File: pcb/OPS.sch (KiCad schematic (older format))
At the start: 45 parts, among them P10 2SC3281, P11 2SC3281, P12 2SA1302, P7 MJE350, P8 MJE340, P9 2SA1302, Q13 MPSA56_PNP_EBC, Q14 MPSA06_NPN_EBC, Q15 MPSA56_PNP_EBC, Q16 MPSA06_NPN_EBC, Q17 MJE340_NPN_ECB, Q18 MJE350_PNP_EBC, Q19 MJE340_NPN_ECB, Q20 MJE350_PNP_EBC

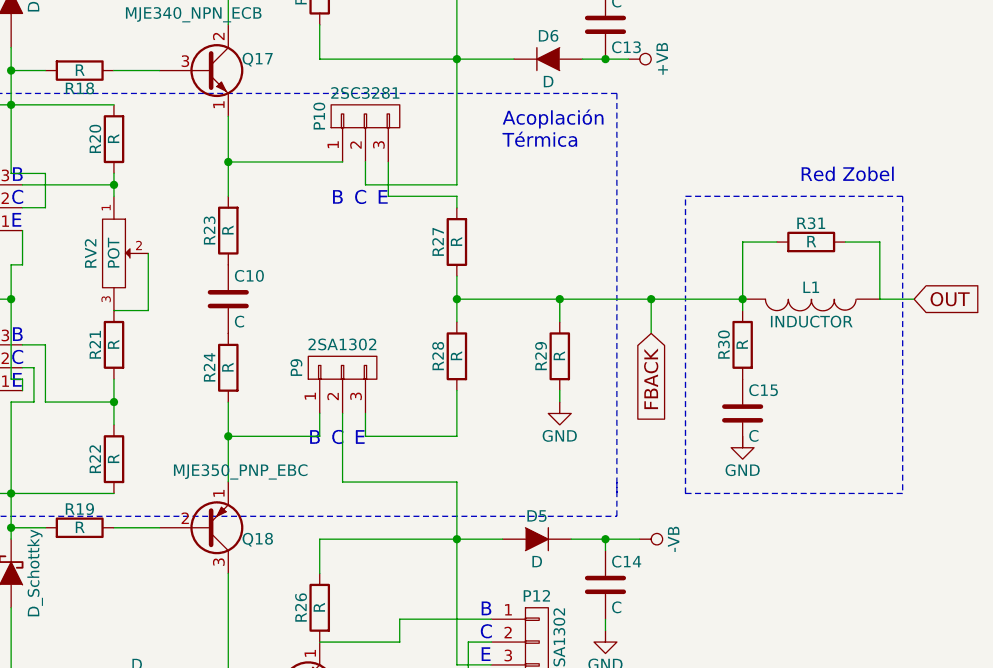
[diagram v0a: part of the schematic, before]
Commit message: ultimos avances falta poco para terminar
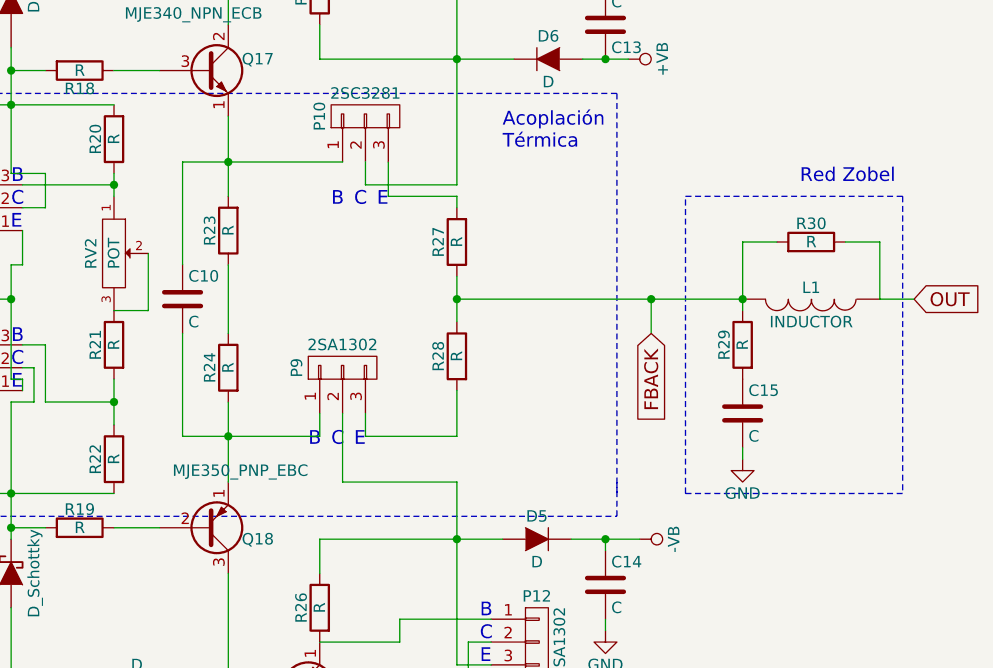
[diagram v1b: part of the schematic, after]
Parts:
- removed R29: R, Resistors_ThroughHole:Resistor_Horizontal_RM10mm, symbol R
- renumbered R30 to R29, R31 to R30
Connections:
- net GND: now also C15.2
- net at R23.1: now also R24.1; no longer C10.1
- net at P10.1 (P1), Q17.1 (E), R23.2: now also C10.1
- net at C10.2: now also P9.1 (P1), Q18.1 (E), R24.2; no longer R24.1
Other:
- moved on the sheet: C10
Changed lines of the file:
@@
 Text GLabel 3450 3550 0    60   Input ~ 0
 TO_OPS
-$Comp
-L R R29
-U 1 1 555E676F
-P 6400 3800
-F 0 "R29" V 6480 3800 50  0000 C CNN
-F 1 "R" V 6400 3800 50  0000 C CNN
-F 2 "Resistors_ThroughHole:Resistor_Horizontal_RM10mm" V 6330 3800 30  0001 C CNN
-F 3 "" H 6400 3800 30  0000 C CNN
-	1    6400 3800
-	-1   0    0    -1
-$EndComp
-$Comp
-L GND #PWR031
-U 1 1 555E69E7
-P 6400 4000
-F 0 "#PWR031" H 6400 3750 50  0001 C CNN
-F 1 "GND" H 6400 3850 50  0000 C CNN
-F 2 "" H 6400 4000 60  0000 C CNN
-F 3 "" H 6400 4000 60  0000 C CNN
-	1    6400 4000
-	1    0    0    -1
-$EndComp
 Text GLabel 6800 3700 3    60   Input ~ 0
 FBACK
 $Comp
-L GND #PWR032
+L GND #PWR031
 U 1 1 555F209B
 P 3200 5050
-F 0 "#PWR032" H 3200 4800 50  0001 C CNN
+F 0 "#PWR031" H 3200 4800 50  0001 C CNN
 F 1 "GND" H 3200 4900 50  0000 C CNN
 F 2 "" H 3200 5050 60  0000 C CNN
@@
 $EndComp
 $Comp
-L GND #PWR033
+L GND #PWR032
 U 1 1 555E698A
 P 3200 2100
-F 0 "#PWR033" H 3200 1850 50  0001 C CNN
+F 0 "#PWR032" H 3200 1850 50  0001 C CNN
 F 1 "GND" H 3200 1950 50  0000 C CNN
 F 2 "" H 3200 2100 60  0000 C CNN
@@
 $EndComp
 $Comp
-L +VA #PWR034
+L +VA #PWR033
 U 1 1 555F2B00
 P 6300 900
-F 0 "#PWR034" H 6300 750 50  0001 C CNN
+F 0 "#PWR033" H 6300 750 50  0001 C CNN
 F 1 "+VA" H 6300 1050 50  0000 C CNN
 F 2 "" H 6300 900 60  0000 C CNN
@@
 $EndComp
 $Comp
-L +VB #PWR035
+L +VB #PWR034
 U 1 1 555F2D0C
 P 6700 2500
-F 0 "#PWR035" H 6700 2350 50  0001 C CNN
+F 0 "#PWR034" H 6700 2350 50  0001 C CNN
 F 1 "+VB" H 6700 2650 50  0000 C CNN
 F 2 "" H 6700 2500 60  0000 C CNN
@@
 $EndComp
 $Comp
-L -VB #PWR036
+L -VB #PWR035
 U 1 1 555F3146
 P 6750 4600
-F 0 "#PWR036" H 6750 4450 50  0001 C CNN
+F 0 "#PWR035" H 6750 4450 50  0001 C CNN
 F 1 "-VB" H 6750 4750 50  0000 C CNN
 F 2 "" H 6750 4600 60  0000 C CNN
@@
 $EndComp
 $Comp
-L -VA #PWR037
+L -VA #PWR036
 U 1 1 555F3328
 P 6300 6200
-F 0 "#PWR037" H 6300 6050 50  0001 C CNN
+F 0 "#PWR036" H 6300 6050 50  0001 C CNN
 F 1 "-VA" H 6300 6350 50  0000 C CNN
 F 2 "" H 6300 6200 60  0000 C CNN
@@
 $EndComp
 $Comp
-L GND #PWR038
+L GND #PWR037
 U 1 1 556CC8CC
 P 5750 5750
-F 0 "#PWR038" H 5750 5500 50  0001 C CNN
+F 0 "#PWR037" H 5750 5500 50  0001 C CNN
 F 1 "GND" H 5750 5600 50  0000 C CNN
 F 2 "" H 5750 5750 60  0000 C CNN
@@
 $EndComp
 $Comp
-L GND #PWR039
+L GND #PWR038
 U 1 1 556CCB94
 P 6150 1300
-F 0 "#PWR039" H 6150 1050 50  0001 C CNN
+F 0 "#PWR038" H 6150 1050 50  0001 C CNN
 F 1 "GND" H 6150 1150 50  0000 C CNN
 F 2 "" H 6150 1300 60  0000 C CNN
@@
 $EndComp
 $Comp
-L GND #PWR040
+L GND #PWR039
 U 1 1 556CECB0
 P 6600 5000
-F 0 "#PWR040" H 6600 4750 50  0001 C CNN
+F 0 "#PWR039" H 6600 4750 50  0001 C CNN
 F 1 "GND" H 6600 4850 50  0000 C CNN
 F 2 "" H 6600 5000 60  0000 C CNN
@@
 $EndComp
 $Comp
-L GND #PWR041
+L GND #PWR040
 U 1 1 556CF118
 P 6600 2200
-F 0 "#PWR041" H 6600 1950 50  0001 C CNN
+F 0 "#PWR040" H 6600 1950 50  0001 C CNN
 F 1 "GND" H 6600 2050 50  0000 C CNN
 F 2 "" H 6600 2200 60  0000 C CNN
@@
 L C C10
 U 1 1 556DE2B0
-P 4950 3550
-F 0 "C10" H 4975 3650 50  0000 L CNN
-F 1 "C" H 4975 3450 50  0000 L CNN
-F 2 "Capacitors_Elko_ThroughHole:Elko_vert_11.5x8mm_RM3.5" H 4988 3400 30  0001 C CNN
-F 3 "" H 4950 3550 60  0000 C CNN
-	1    4950 3550
-	1    0    0    -1
-$EndComp
-$Comp
-L R R30
+P 4750 3550
+F 0 "C10" H 4775 3650 50  0000 L CNN
+F 1 "C" H 4775 3450 50  0000 L CNN
+F 2 "Capacitors_Elko_ThroughHole:Elko_vert_11.5x8mm_RM3.5" H 4788 3400 30  0001 C CNN
+F 3 "" H 4750 3550 60  0000 C CNN
+	1    4750 3550
+	1    0    0    -1
+$EndComp
+$Comp
+L R R29
 U 1 1 556E028A
 P 7200 3750
-F 0 "R30" V 7280 3750 50  0000 C CNN
+F 0 "R29" V 7280 3750 50  0000 C CNN
 F 1 "R" V 7200 3750 50  0000 C CNN
 F 2 "Resistors_ThroughHole:Resistor_Horizontal_RM10mm" V 7130 3750 30  0001 C CNN
@@
 $EndComp
 $Comp
-L R R31
+L R R30
 U 1 1 556E05E0
 P 7500 3300
-F 0 "R31" V 7580 3300 50  0000 C CNN
+F 0 "R30" V 7580 3300 50  0000 C CNN
 F 1 "R" V 7500 3300 50  0000 C CNN
 F 2 "Resistors_ThroughHole:Resistor_Horizontal_RM10mm" V 7430 3300 30  0001 C CNN
@@
 OUT
 $Comp
-L GND #PWR042
+L GND #PWR041
 U 1 1 556E0BD9
-P 7200 4150
-F 0 "#PWR042" H 7200 3900 50  0001 C CNN
-F 1 "GND" H 7200 4000 50  0000 C CNN
-F 2 "" H 7200 4150 60  0000 C CNN
-F 3 "" H 7200 4150 60  0000 C CNN
-	1    7200 4150
+P 7200 4250
+F 0 "#PWR041" H 7200 4000 50  0001 C CNN
+F 1 "GND" H 7200 4100 50  0000 C CNN
+F 2 "" H 7200 4250 60  0000 C CNN
+F 3 "" H 7200 4250 60  0000 C CNN
+	1    7200 4250
 	1    0    0    -1
 $EndComp
@@
 	5350 4150 5350 4050
 Wire Wire Line
-	4950 4150 5350 4150
+	4750 4150 5350 4150
 Wire Wire Line
 	5550 3050 5550 2950
@@
 	5950 3150 5950 3100
 Wire Wire Line
-	4950 2950 5450 2950
+	4750 2950 5450 2950
 Wire Wire Line
 	4150 3750 4150 4000
@@
 	4000 3400 4050 3400
 Wire Wire Line
-	6400 3950 6400 4000
-Wire Wire Line
 	3200 2100 3200 2050
-Connection ~ 6400 3550
-Wire Wire Line
-	6400 3550 6400 3650
 Connection ~ 5950 3550
 Wire Wire Line
@@
 Wire Wire Line
 	3200 1550 3200 1750
+Wire Wire Line
+	4750 3400 4750 2950
+Wire Wire Line
+	4750 3700 4750 4150
+Wire Wire Line
+	4950 3700 4950 3400
+Wire Wire Line
+	7200 4200 7200 4250
 $EndSCHEMATC
